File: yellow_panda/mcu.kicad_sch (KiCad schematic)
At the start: 32 parts, among them SW65 SW_SPDT, SW66 SW_SPDT, SW67 SW_Push, SW68 SW_Push, U3 STM32F446RCTx, U4 STM32F446RCTx, Y1 8MHz, Y2 8MHz

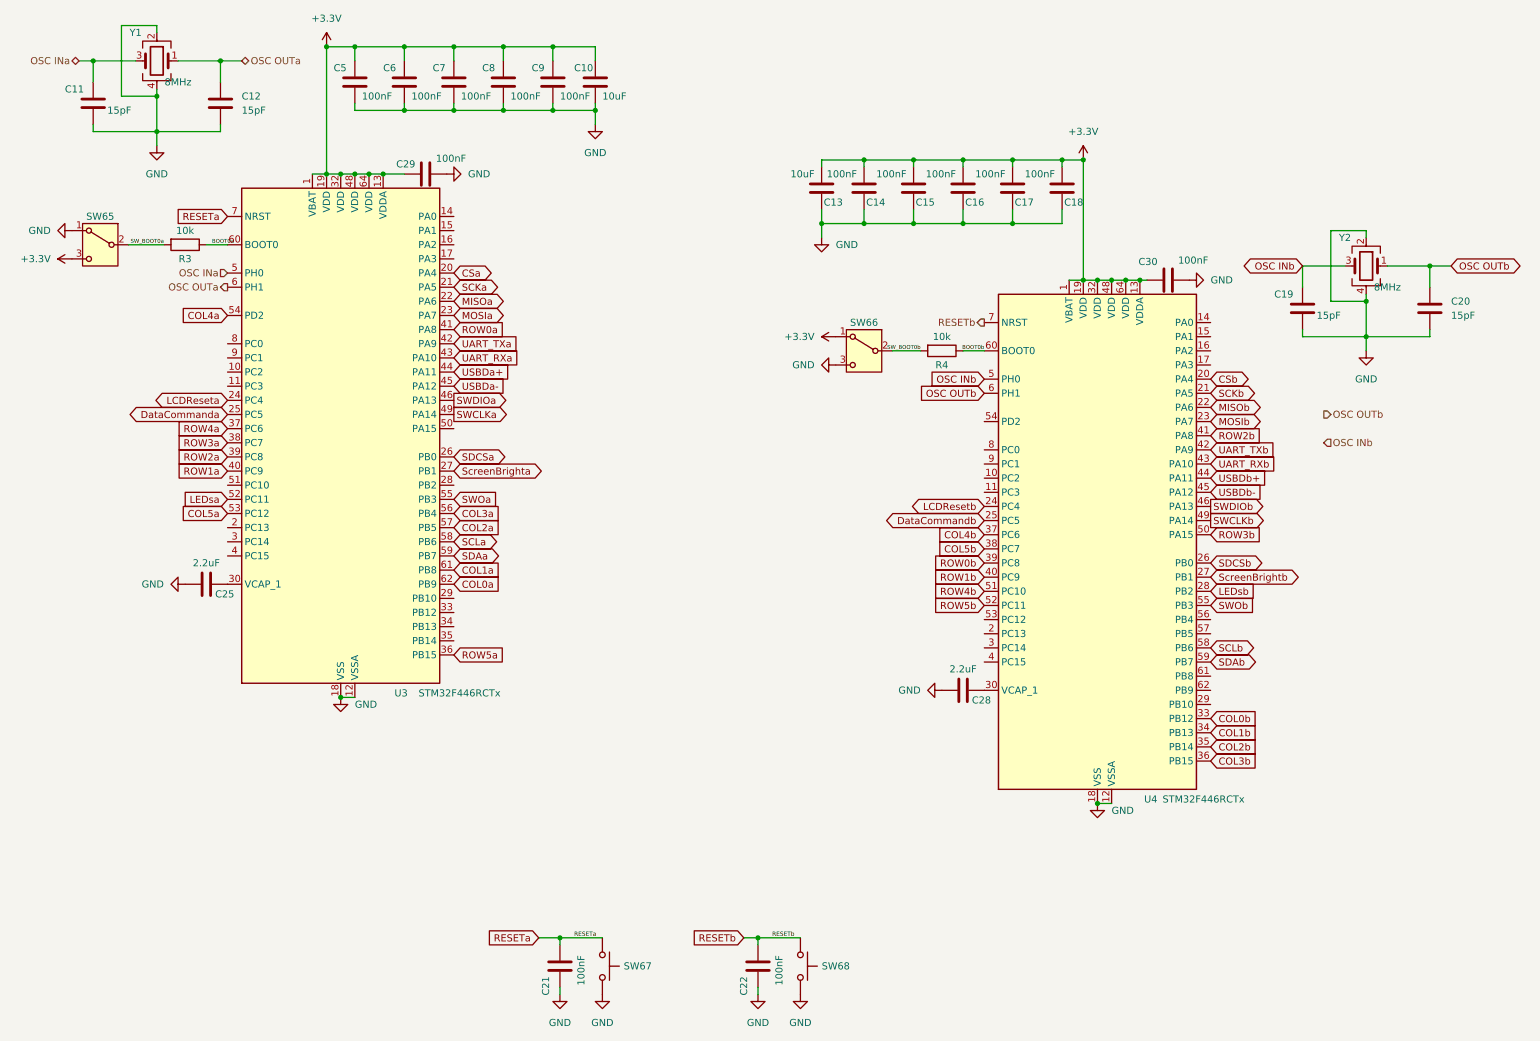
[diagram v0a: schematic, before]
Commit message: v0.1b
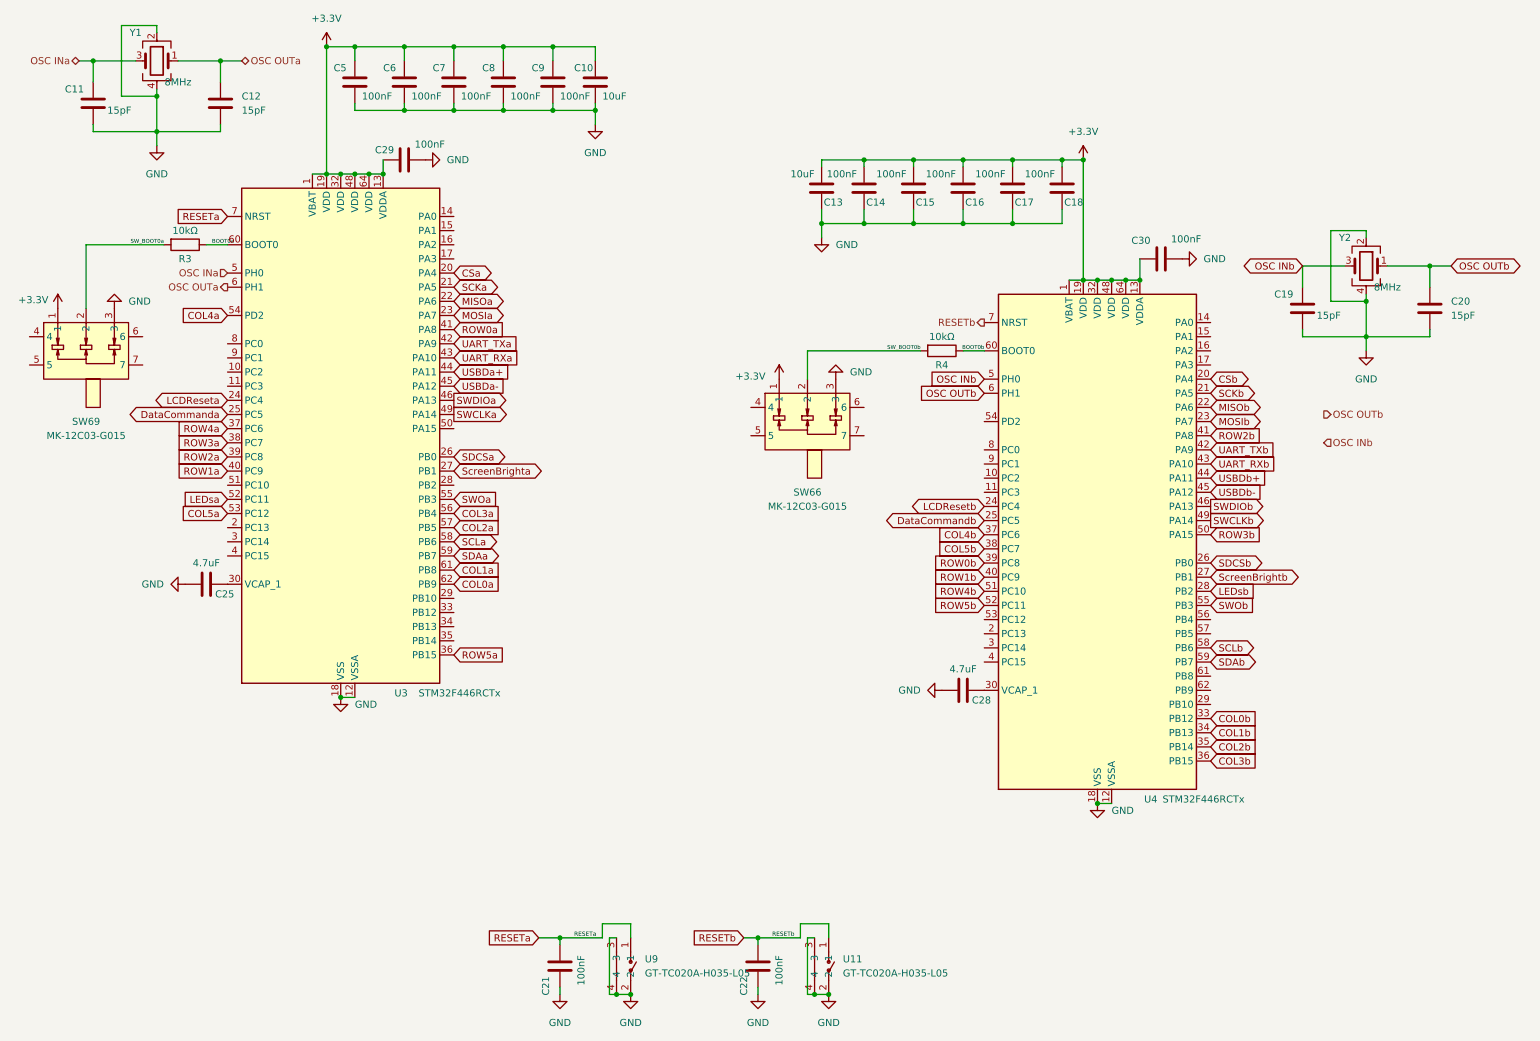
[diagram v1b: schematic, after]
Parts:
- removed SW65, SW66: SW_SPDT, Custom Lib:SLW-66527511-SMT-TR_CUD, symbol Switch:SW_SPDT
- removed SW67, SW68: SW_Push, Custom Lib:SW_TL3330_EWI, symbol Switch:SW_Push
- added SW66, SW69: MK-12C03-G015, easyeda2kicad:SW-SMD_MK-12C03-G015, symbol easyeda2kicad:MK-12C03-G015
- added U11, U9: GT-TC020A-H035-L05, easyeda2kicad:SW-SMD_GT-TC020B-H035-L05, symbol easyeda2kicad:GT-TC020A-H035-L05
- C10, C13: footprint Capacitor_SMD:C_1206_3216Metric_Pad1.33x1.80mm_HandSolder -> Capacitor_SMD:C_1206_3216Metric; LCSC (none) -> C13585; LCSC Part (none) -> C13585
- C11, C12, C19, C20: footprint Capacitor_SMD:C_0402_1005Metric_Pad0.74x0.62mm_HandSolder -> Capacitor_SMD:C_0402_1005Metric; LCSC (none) -> C441742; LCSC Part (none) -> C441742
- C14, C15, C16, C17, C18, C21, C22, C29, C30, C5, C6, C7, C8, C9: footprint Capacitor_SMD:C_0201_0603Metric_Pad0.64x0.40mm_HandSolder -> Capacitor_SMD:C_0805_2012Metric; LCSC (none) -> C48579599; LCSC Part (none) -> C48579599
- C25, C28: value 2.2uF -> 4.7uF; footprint Capacitor_SMD:C_0603_1608Metric_Pad1.08x0.95mm_HandSolder -> Capacitor_SMD:C_0603_1608Metric; LCSC (none) -> C1705; LCSC Part (none) -> C1705
- R3, R4: value 10k -> 10kΩ; footprint Resistor_SMD:R_0402_1005Metric_Pad0.72x0.64mm_HandSolder -> Resistor_SMD:R_0805_2012Metric; LCSC (none) -> C84376; LCSC Part (none) -> C84376
- U3, U4: LCSC (none) -> C915971; LCSC Part (none) -> C915971
- Y1, Y2: LCSC (none) -> C1985378; LCSC Part (none) -> C1985378
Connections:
- net +3.3V: now also SW66.1, SW69.1
- net GND: now also SW66.3, SW69.3, U11.2, U11.3, U11.4, U9.2, U9.3, U9.4
- net RESETa: now also U9.1
- net RESETb: now also U11.1
- net SW_BOOT0a: now also SW69.2
- net SW_BOOT0b: now also SW66.2
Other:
- moved on the sheet: C29, C30

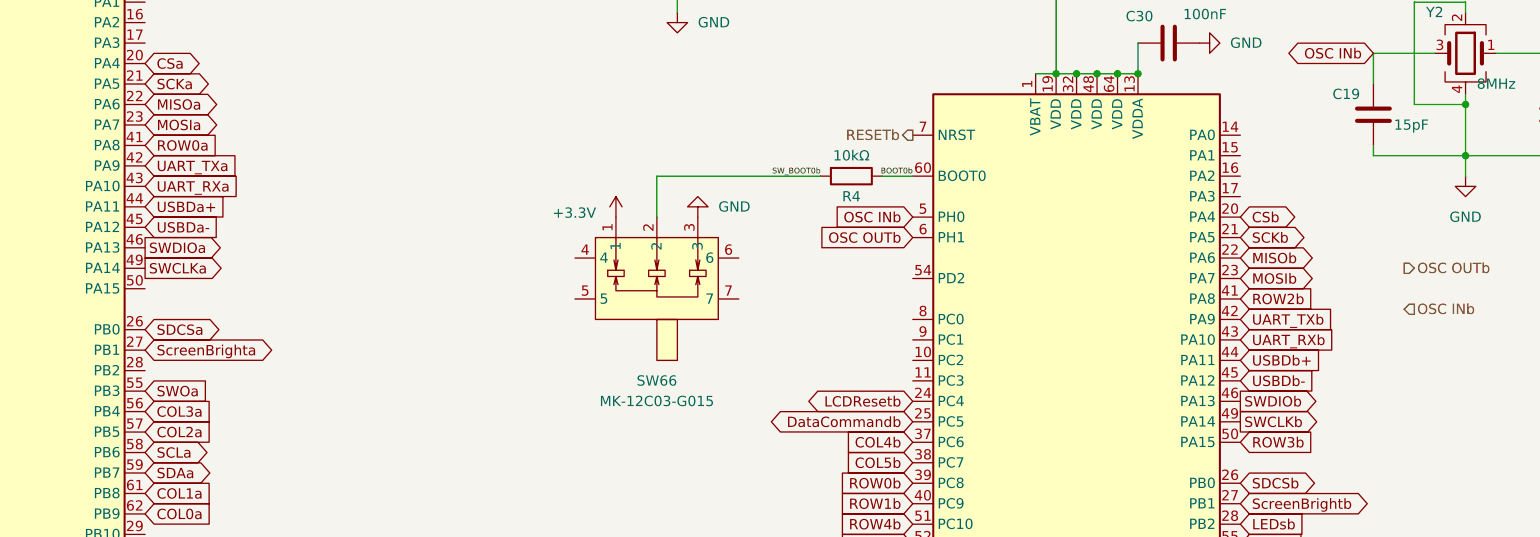
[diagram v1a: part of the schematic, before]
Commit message: v1.0a
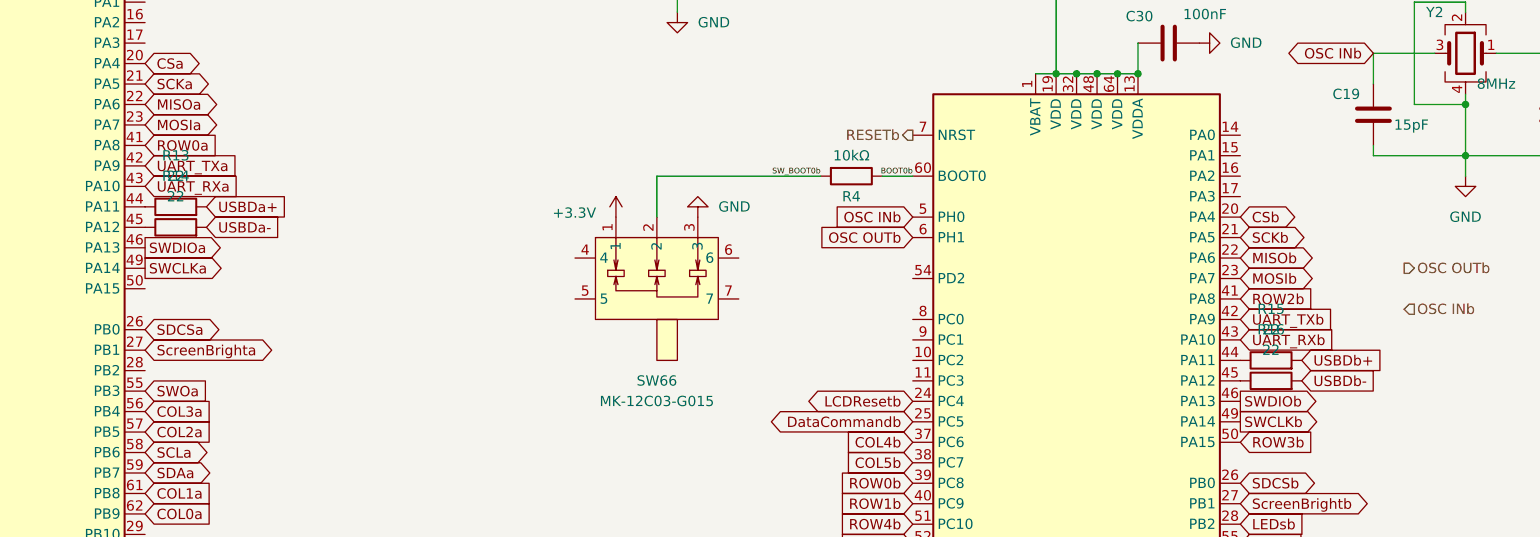
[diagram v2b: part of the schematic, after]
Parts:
- added R13, R14, R15, R16: 22, Resistor_SMD:R_0402_1005Metric, symbol Device:R
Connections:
- net USBDa+: now also R13.2; no longer U3.44 (PA11)
- net USBDa-: now also R14.2; no longer U3.45 (PA12)
- net USBDb+: now also R15.2; no longer U4.44 (PA11)
- net USBDb-: now also R16.2; no longer U4.45 (PA12)
- new net: R15.1, U4.44 (PA11)
- new net: R14.1, U3.45 (PA12)
- new net: R13.1, U3.44 (PA11)
- new net: R16.1, U4.45 (PA12)
